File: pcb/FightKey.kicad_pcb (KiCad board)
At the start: 2 copper layers, 201.9 x 85.1 mm, 29 parts, among them J1 Conn_01x016_Male

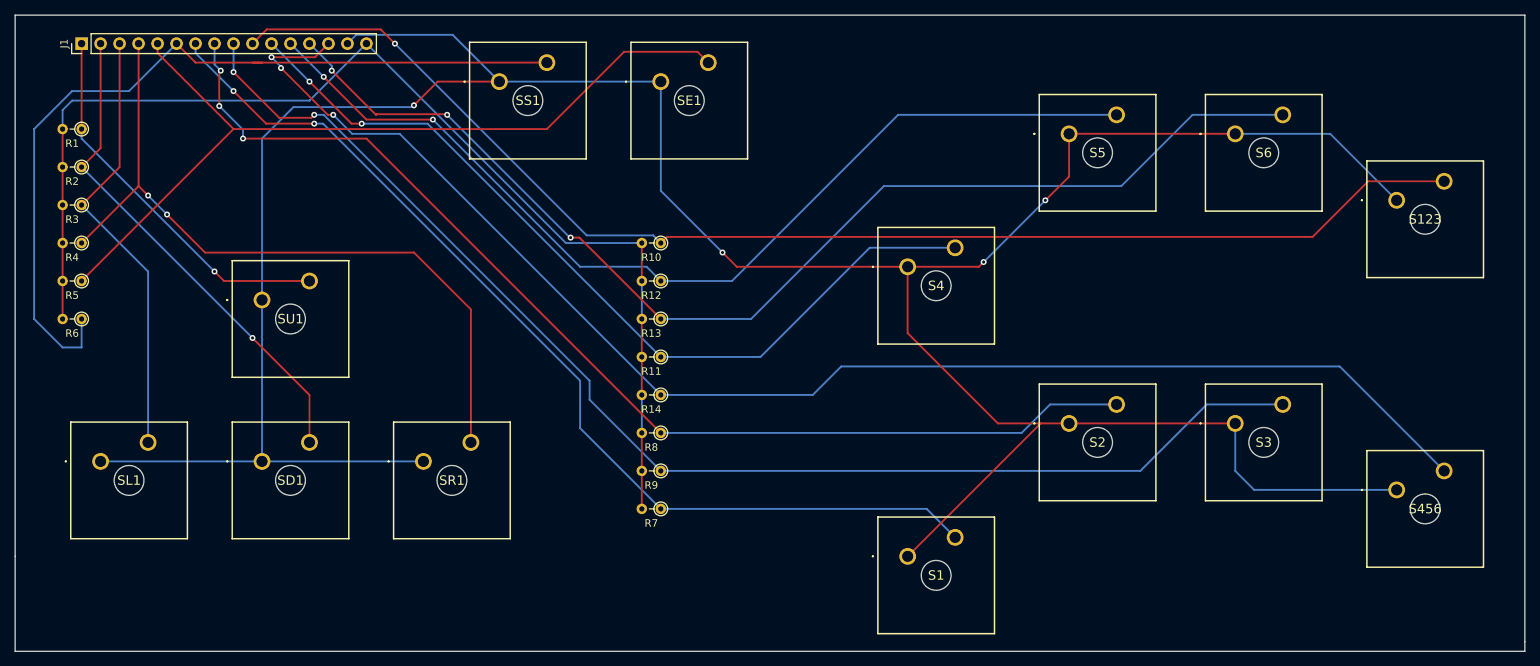
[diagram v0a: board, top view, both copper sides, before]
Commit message: Added enclosure and final picture
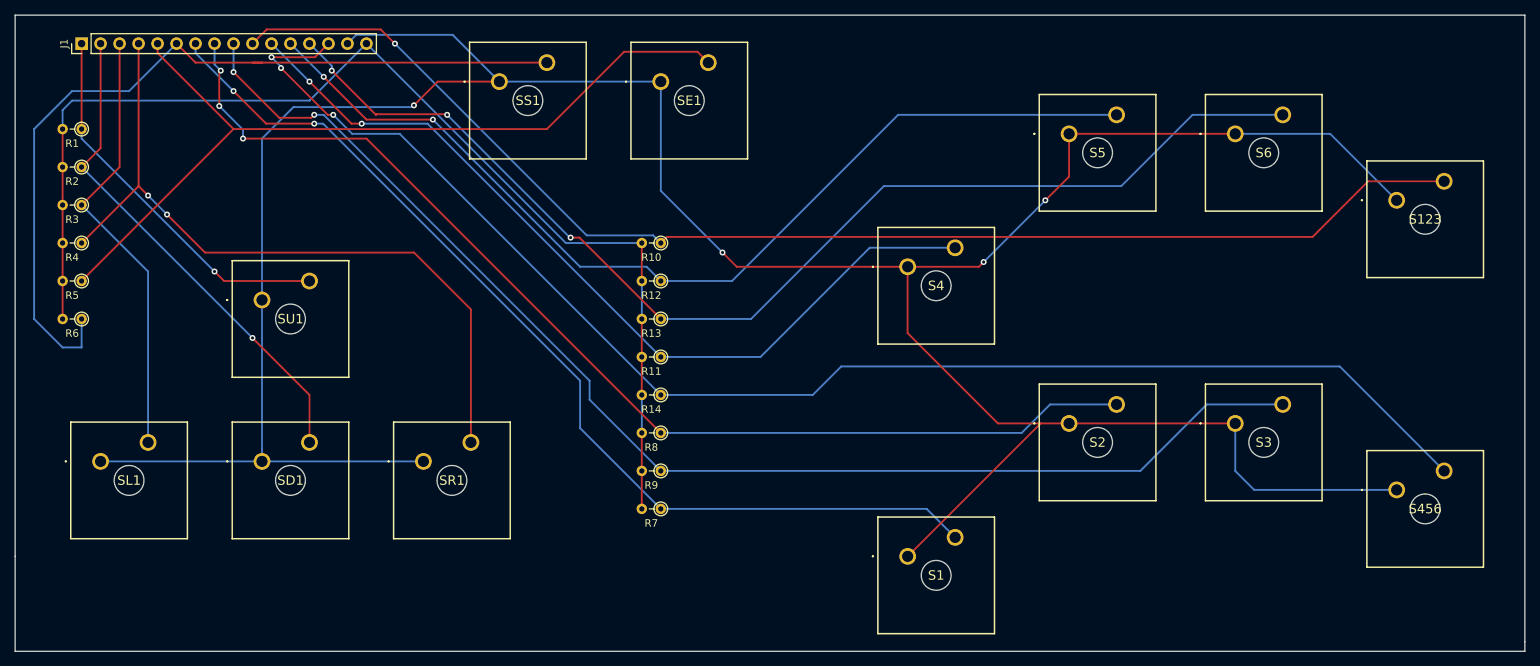
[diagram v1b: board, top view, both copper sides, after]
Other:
- net class Default removed
